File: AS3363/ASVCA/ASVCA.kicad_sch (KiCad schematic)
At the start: 18 parts

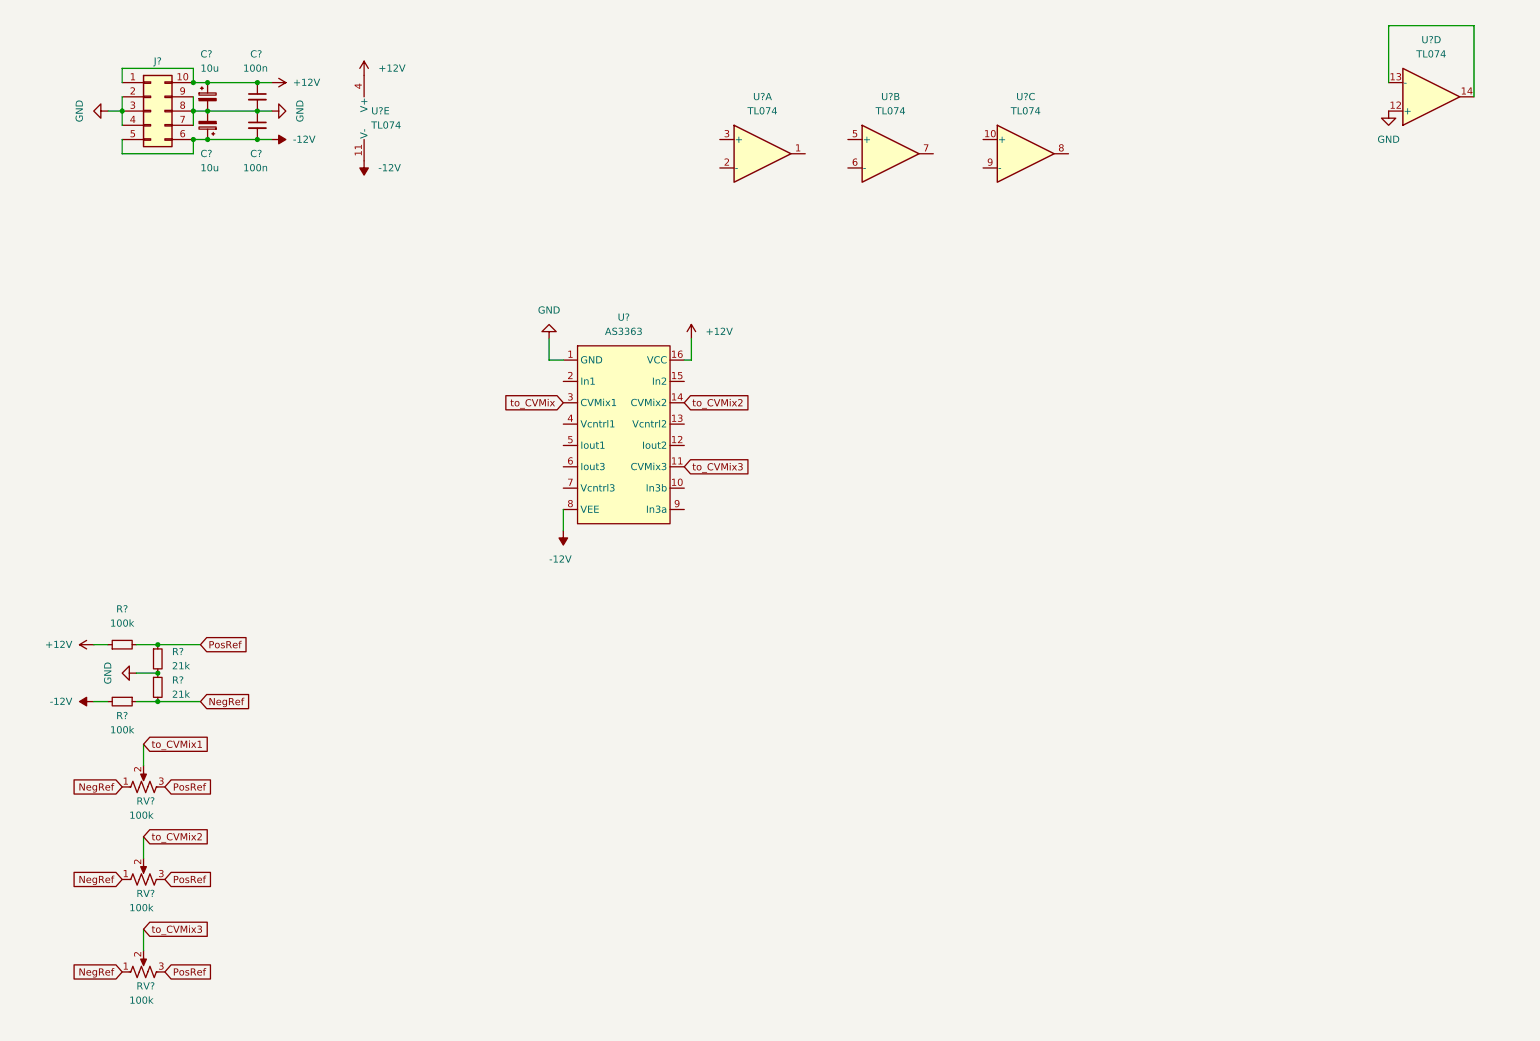
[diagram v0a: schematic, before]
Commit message: 123
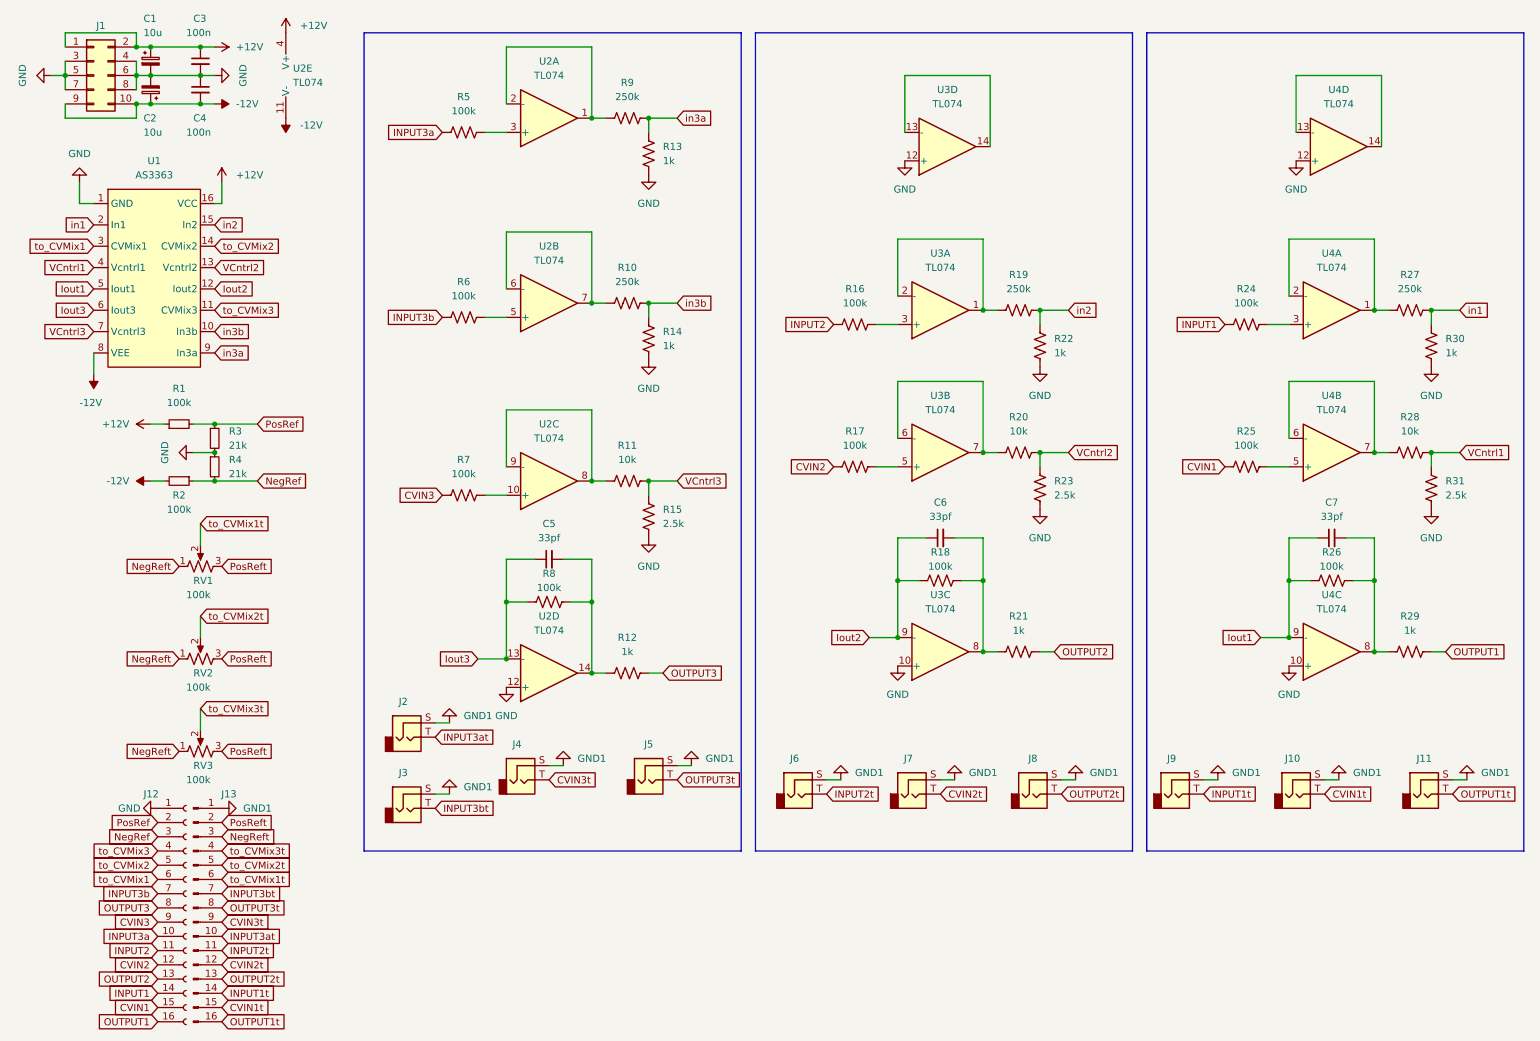
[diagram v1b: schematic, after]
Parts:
- added C5, C6, C7: 33pf, Capacitor_THT:C_Disc_D6.0mm_W2.5mm_P5.00mm, symbol Device:C_Small
- added J10: CVIN1, benjiaomodular:AudioJack_3.5mm, symbol Connector:AudioJack2
- added J11: OUTPUT1, benjiaomodular:AudioJack_3.5mm, symbol Connector:AudioJack2
- added J12: Conn_01x14_Female, Connector_PinHeader_2.54mm:PinHeader_1x16_P2.54mm_Vertical, symbol Connector:Conn_01x16_Female
- added J13: Conn_01x14_Male, Connector_PinHeader_2.54mm:PinHeader_1x16_P2.54mm_Vertical, symbol Connector:Conn_01x16_Male
- added J2: INPUT3a, benjiaomodular:AudioJack_3.5mm, symbol Connector:AudioJack2
- added J3: INPUT3b, benjiaomodular:AudioJack_3.5mm, symbol Connector:AudioJack2
- added J4: CVIN3, benjiaomodular:AudioJack_3.5mm, symbol Connector:AudioJack2
- added J5: OUTPUT3, benjiaomodular:AudioJack_3.5mm, symbol Connector:AudioJack2
- added J6: INPUT2, benjiaomodular:AudioJack_3.5mm, symbol Connector:AudioJack2
- added J7: CVIN2, benjiaomodular:AudioJack_3.5mm, symbol Connector:AudioJack2
- added J8: OUTPUT2, benjiaomodular:AudioJack_3.5mm, symbol Connector:AudioJack2
- added J9: INPUT1, benjiaomodular:AudioJack_3.5mm, symbol Connector:AudioJack2
- added R10, R19, R27, R9: 250k, benjiaomodular:Resistor_L6.3mm_D2.5mm_P7.62mm_Horizontal, symbol Device:R_US
- added R11, R20, R28: 10k, benjiaomodular:Resistor_L6.3mm_D2.5mm_P7.62mm_Horizontal, symbol Device:R_US
- added R12, R13, R14, R21, R22, R29, R30: 1k, benjiaomodular:Resistor_L6.3mm_D2.5mm_P7.62mm_Horizontal, symbol Device:R_US
- added R15, R23, R31: 2.5k, benjiaomodular:Resistor_L6.3mm_D2.5mm_P7.62mm_Horizontal, symbol Device:R_US
- added R16, R17, R18, R24, R25, R26, R5, R6, R7, R8: 100k, benjiaomodular:Resistor_L6.3mm_D2.5mm_P7.62mm_Horizontal, symbol Device:R_US
- added unit 1 of U2
- added unit 2 of U2
- added unit 4 of U2
- added unit 3 of U2
- added U3: TL074, Package_DIP:DIP-14_W7.62mm_Socket, symbol Amplifier_Operational:TL074
- C1, C2: renamed from C?; footprint (none) -> Capacitor_THT:CP_Radial_D5.0mm_P2.50mm
- C3, C4: renamed from C?; footprint (none) -> Capacitor_THT:C_Disc_D6.0mm_W2.5mm_P5.00mm
- J1: renamed from J?; footprint (none) -> Connector_IDC:IDC-Header_2x05_P2.54mm_Vertical; symbol Connector_Generic:Conn_02x05_Counter_Clockwise -> Connector_Generic:Conn_02x05_Odd_Even
- R1, R2, R3, R4: renamed from R?; footprint (none) -> benjiaomodular:Resistor_L6.3mm_D2.5mm_P7.62mm_Horizontal
- RV1, RV2, RV3: renamed from RV?; footprint (none) -> benjiaomodular:Potentiometer_RV09
- U1: renamed from U?; footprint (none) -> Package_DIP:DIP-16_W7.62mm_Socket
- U2, U4: renamed from U?; footprint (none) -> Package_DIP:DIP-14_W7.62mm_Socket
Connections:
- net to_CVMix is gone; now on net to_CVMix1: U1.3 (CVMix1)
- net +12V: now also J1.2 (Pin_2); no longer J1.10 (Pin_10)
- net -12V: now also J1.10 (Pin_10), J1.9 (Pin_9); no longer J1.5 (Pin_5), J1.6 (Pin_6)
- net GND: now also J1.5 (Pin_5), J1.6 (Pin_6), U4.10 (+), J12.1 (Pin_1), R13.1, R14.1, R15.1, R22.1, R23.1, R30.1, R31.1, U2.12 (+), U3.10 (+), U3.12 (+); no longer J1.2 (Pin_2), J1.9 (Pin_9)
- net NegRef: now also J12.3 (Pin_3); no longer RV1.1, RV2.1, RV3.1
- net PosRef: now also J12.2 (Pin_2); no longer RV1.3, RV2.3, RV3.3
- net to_CVMix1: now also J12.6 (Pin_6); no longer RV1.2
- net to_CVMix2: now also J12.5 (Pin_5); no longer RV2.2
- net to_CVMix3: now also J12.4 (Pin_4); no longer RV3.2
- net in3b: now reaches U1.10 (In3b)
- net in3b: now also R10.2, R14.2
- net Iout2: now reaches U1.12 (Iout2)
- net Iout2: now also C6.1, R18.1, U3.9 (-)
- net VCntrl2: now reaches U1.13 (Vcntrl2)
- net VCntrl2: now also R20.2, R23.2
- net in2: now reaches U1.15 (In2)
- net in2: now also R19.2, R22.2
- net in1: now reaches U1.2 (In1)
- net in1: now also R27.2, R30.2
- net VCntrl1: now reaches U1.4 (Vcntrl1)
- net VCntrl1: now also R28.2, R31.2
- net Iout1: now reaches U1.5 (Iout1)
- net Iout1: now also U4.9 (-), C7.1, R26.1
- net Iout3: now reaches U1.6 (Iout3)
- net Iout3: now also C5.1, R8.1, U2.13 (-)
- net VCntrl3: now reaches U1.7 (Vcntrl3)
- net VCntrl3: now also R11.2, R15.2
- net in3a: now reaches U1.9 (In3a)
- net in3a: now also R13.2, R9.2
- net at U4.5 (+): now also R25.2
- net at U4.6 (-): now also U4.7, R28.1
- net at U4.8: now also C7.2, R26.2, R29.2
- net at U4.1: now also U4.2 (-), R27.1
- net at U4.3 (+): now also R24.2
- new net: R17.2, U3.5 (+)
- new net: R20.1, U3.6 (-), U3.7
- new net: C6.2, R18.2, R21.2, U3.8
- new net: U3.13 (-), U3.14
- new net: R6.2, U2.5 (+)
- new net: R19.1, U3.1, U3.2 (-)
- new net: R5.2, U2.3 (+)
- new net: R9.1, U2.1, U2.2 (-)
- new net: R11.1, U2.8, U2.9 (-)
- new net: C5.2, R12.2, R8.2, U2.14
- new net: R16.2, U3.3 (+)
- new net: R10.1, U2.6 (-), U2.7
- new net: R7.2, U2.10 (+)
- new net CVIN1: J12.15 (Pin_15), R25.1
- new net CVIN1t: J10.T, J13.15 (Pin_15)
- new net CVIN2: J12.12 (Pin_12), R17.1
- new net CVIN2t: J13.12 (Pin_12), J7.T
- new net CVIN3: J12.9 (Pin_9), R7.1
- new net CVIN3t: J13.9 (Pin_9), J4.T
- new net GND1: J10.S, J11.S, J13.1 (Pin_1), J2.S, J3.S, J4.S, J5.S, J6.S, J7.S, J8.S, J9.S
- new net INPUT1: J12.14 (Pin_14), R24.1
- new net INPUT1t: J13.14 (Pin_14), J9.T
- new net INPUT2: J12.11 (Pin_11), R16.1
- new net INPUT2t: J13.11 (Pin_11), J6.T
- new net INPUT3a: J12.10 (Pin_10), R5.1
- new net INPUT3at: J13.10 (Pin_10), J2.T
- new net INPUT3b: J12.7 (Pin_7), R6.1
- new net INPUT3bt: J13.7 (Pin_7), J3.T
- new net NegReft: J13.3 (Pin_3), RV1.1, RV2.1, RV3.1
- new net OUTPUT1: J12.16 (Pin_16), R29.1
- new net OUTPUT1t: J11.T, J13.16 (Pin_16)
- new net OUTPUT2: J12.13 (Pin_13), R21.1
- new net OUTPUT2t: J13.13 (Pin_13), J8.T
- new net OUTPUT3: J12.8 (Pin_8), R12.1
- new net OUTPUT3t: J13.8 (Pin_8), J5.T
- new net PosReft: J13.2 (Pin_2), RV1.3, RV2.3, RV3.3
- new net to_CVMix1t: J13.6 (Pin_6), RV1.2
- new net to_CVMix2t: J13.5 (Pin_5), RV2.2
- new net to_CVMix3t: J13.4 (Pin_4), RV3.2
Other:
- moved on the sheet: C1, C2, C3, C4, J1, R1, R2, R3, R4, RV1, RV2, RV3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
